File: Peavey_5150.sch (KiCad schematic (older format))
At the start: 203 parts, among them J165 SEND, J166 RETURN, J2 Power, J3 OUTPUT, J37 INPUT FRONT, J39 INPUT REAR, J4 SWIM, J5 FOOTSWITCH, K1 G5V-2, K2 G5V-2, K3 G5V-2, K4 G5V-2, K5 G5V1, Q1 IRF840, Q2 BC847, Q3 BC847, Q4 BC847, SW2 Clean, SW3 Bright, SW4 FX_loop, U1 MP4462, U2 AMS1117-3.3, U3 STM8S003F3P, U4 TLP222A

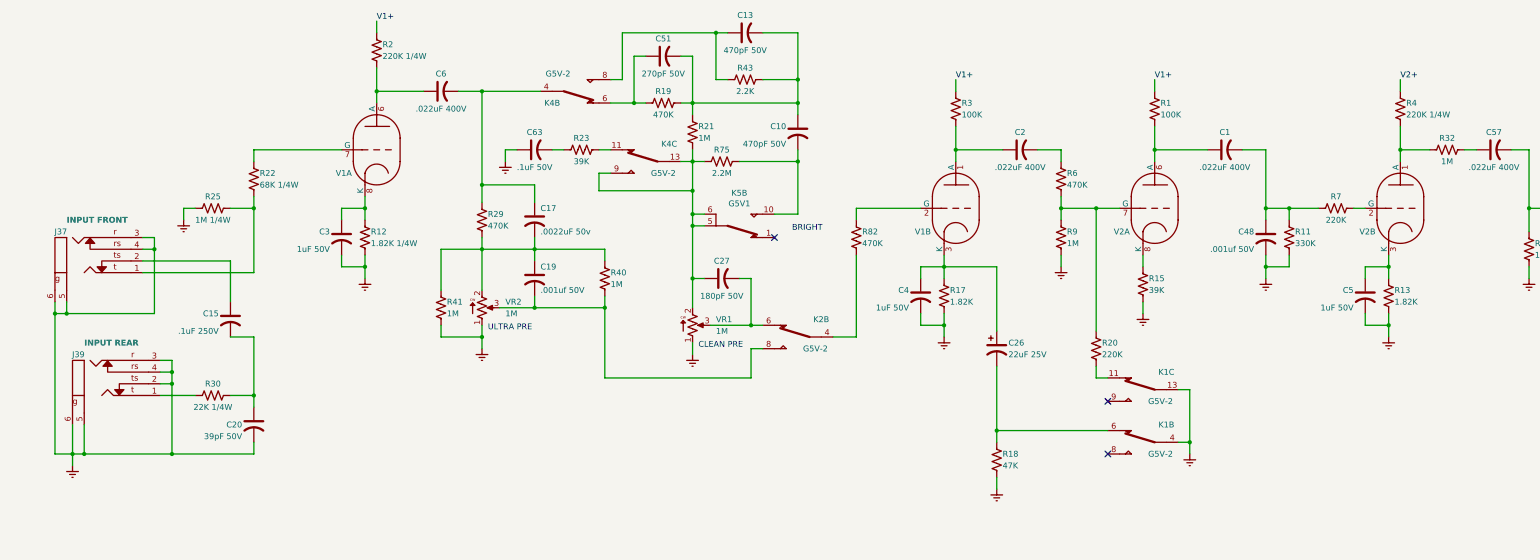
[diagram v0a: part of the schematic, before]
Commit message: add some r watts
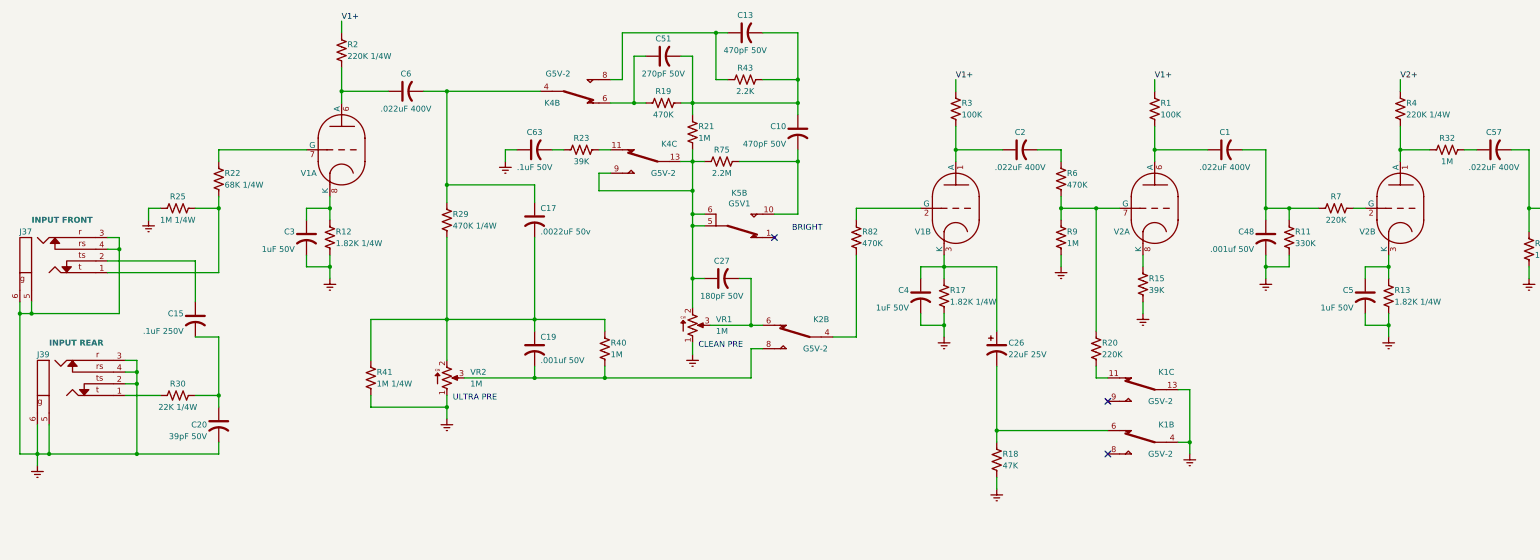
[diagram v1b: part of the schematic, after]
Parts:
- R13, R17: value 1.82K -> 1.82K 1/4W
- R29: value 470K -> 470K 1/4W
- R41: value 1M -> 1M 1/4W
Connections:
- wire segments 724 -> 723
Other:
- moved on the sheet: C15, C19, C20, C3, C6, J37, J39, R12, R2, R22, R25, R29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
